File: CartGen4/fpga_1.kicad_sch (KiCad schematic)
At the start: 4 parts, among them U9 LFXP2-8E-5MN132C

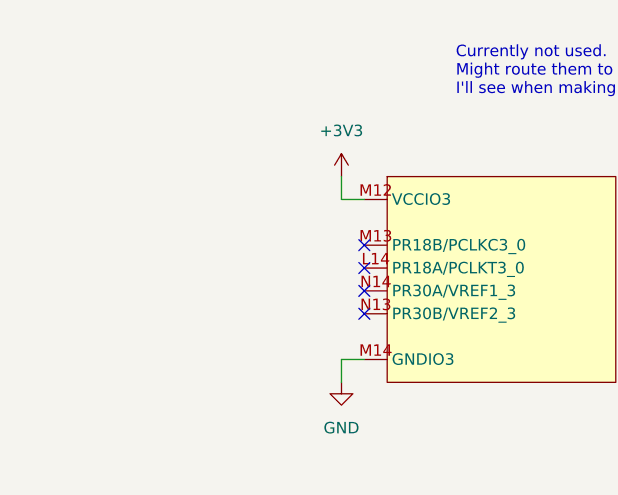
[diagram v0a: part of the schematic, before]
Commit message: Fixed DRC
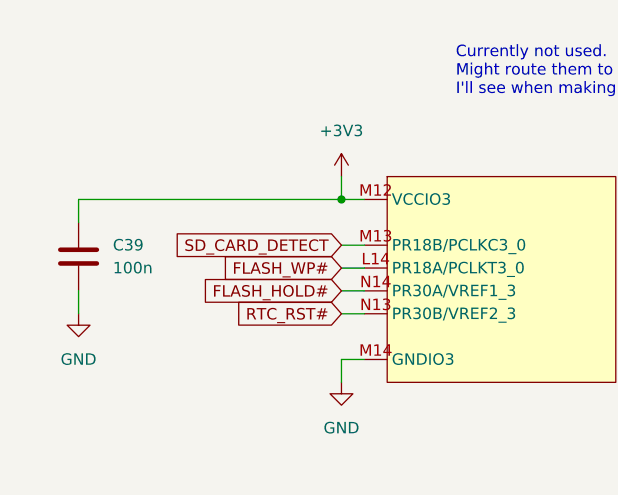
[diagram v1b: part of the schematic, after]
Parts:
- added C39: 100n, symbol Device:C
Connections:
- net +3V3: now also C39.1
- net GND: now also C39.2
- net FLASH_WP#: now reaches U9.L14 (PR18A/PCLKT3_0)
- net SD_CARD_DETECT: now reaches U9.M13 (PR18B/PCLKC3_0)
- net RTC_RST#: now reaches U9.N13 (PR30B/VREF2_3)
- net FLASH_HOLD#: now reaches U9.N14 (PR30A/VREF1_3)
- no-connect marks 8 -> 4
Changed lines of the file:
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@@
   (junction (at 60.96 33.02) (diameter 0) (color 0 0 0 0)
   )
+  (junction (at 50.8 143.51) (diameter 0) (color 0 0 0 0)
+  )
   (junction (at 139.7 48.26) (diameter 0) (color 0 0 0 0)
   )
-  (no_connect (at 53.34 156.21))
   (no_connect (at 119.38 156.21))
   (no_connect (at 119.38 153.67))
   (no_connect (at 119.38 151.13))
   (no_connect (at 119.38 148.59))
-  (no_connect (at 53.34 148.59))
-  (no_connect (at 53.34 151.13))
-  (no_connect (at 53.34 153.67))
   (bus_entry (at 46.99 73.66) (size 2.54 2.54)
     (stroke (width 0) (type default) (color 0 0 0 0))
@@
     (stroke (width 0) (type default) (color 0 0 0 0))
   )
+  (wire (pts (xy 21.59 153.67) (xy 21.59 156.21))
+    (stroke (width 0) (type default) (color 0 0 0 0))
+  )
   (bus (pts (xy 125.73 55.88) (xy 125.73 53.34))
     (stroke (width 0) (type default) (color 0 0 0 0))
@@
     (stroke (width 0) (type default) (color 0 0 0 0))
   )
+  (wire (pts (xy 21.59 143.51) (xy 50.8 143.51))
+    (stroke (width 0) (type default) (color 0 0 0 0))
+  )
   (wire (pts (xy 128.27 81.28) (xy 142.24 81.28))
     (stroke (width 0) (type default) (color 0 0 0 0))
@@
     (stroke (width 0) (type default) (color 0 0 0 0))
   )
+  (wire (pts (xy 50.8 153.67) (xy 53.34 153.67))
+    (stroke (width 0) (type default) (color 0 0 0 0))
+  )
   (wire (pts (xy 128.27 55.88) (xy 142.24 55.88))
     (stroke (width 0) (type default) (color 0 0 0 0))
@@
     (stroke (width 0) (type default) (color 0 0 0 0))
   )
+  (wire (pts (xy 21.59 146.05) (xy 21.59 143.51))
+    (stroke (width 0) (type default) (color 0 0 0 0))
+  )
   (wire (pts (xy 148.59 25.4) (xy 139.7 25.4))
     (stroke (width 0) (type default) (color 0 0 0 0))
@@
     (stroke (width 0) (type default) (color 0 0 0 0))
   )
+  (wire (pts (xy 50.8 151.13) (xy 53.34 151.13))
+    (stroke (width 0) (type default) (color 0 0 0 0))
+  )
   (wire (pts (xy 223.52 69.85) (xy 226.06 69.85))
     (stroke (width 0) (type default) (color 0 0 0 0))
@@
     (stroke (width 0) (type default) (color 0 0 0 0))
   )
+  (wire (pts (xy 50.8 148.59) (xy 53.34 148.59))
+    (stroke (width 0) (type default) (color 0 0 0 0))
+  )
   (bus (pts (xy 125.73 76.2) (xy 125.73 73.66))
     (stroke (width 0) (type default) (color 0 0 0 0))
@@
   )
   (wire (pts (xy 53.34 161.29) (xy 50.8 161.29))
+    (stroke (width 0) (type default) (color 0 0 0 0))
+  )
+  (wire (pts (xy 50.8 156.21) (xy 53.34 156.21))
     (stroke (width 0) (type default) (color 0 0 0 0))
   )
@@
     )
   )
+  (global_label "FLASH_WP#" (shape input) (at 50.8 151.13 180) (fields_autoplaced)
+    (effects (font (size 1.27 1.27)) (justify right))
+    (property "Intersheet References" "${INTERSHEET_REFS}" (id 0) (at 37.6826 151.0506 0)
+      (effects (font (size 1.27 1.27)) (justify right) hide)
+    )
+  )
   (global_label "GB_DATA[0..7]" (shape input) (at 34.29 55.88 180) (fields_autoplaced)
     (effects (font (size 1.27 1.27)) (justify right))
@@
     )
   )
+  (global_label "RTC_RST#" (shape input) (at 50.8 156.21 180) (fields_autoplaced)
+    (effects (font (size 1.27 1.27)) (justify right))
+    (property "Intersheet References" "${INTERSHEET_REFS}" (id 0) (at 39.1945 156.1306 0)
+      (effects (font (size 1.27 1.27)) (justify right) hide)
+    )
+  )
   (global_label "GB_RD#" (shape input) (at 223.52 69.85 180) (fields_autoplaced)
     (effects (font (size 1.27 1.27)) (justify right))
@@
     (effects (font (size 1.27 1.27)) (justify right))
     (property "Intersheet References" "${INTERSHEET_REFS}" (id 0) (at 177.0198 51.9906 0)
+      (effects (font (size 1.27 1.27)) (justify right) hide)
+    )
+  )
+  (global_label "FLASH_HOLD#" (shape input) (at 50.8 153.67 180) (fields_autoplaced)
+    (effects (font (size 1.27 1.27)) (justify right))
+    (property "Intersheet References" "${INTERSHEET_REFS}" (id 0) (at 35.445 153.5906 0)
+      (effects (font (size 1.27 1.27)) (justify right) hide)
+    )
+  )
+  (global_label "SD_CARD_DETECT" (shape input) (at 50.8 148.59 180) (fields_autoplaced)
+    (effects (font (size 1.27 1.27)) (justify right))
+    (property "Intersheet References" "${INTERSHEET_REFS}" (id 0) (at 32.3002 148.6694 0)
       (effects (font (size 1.27 1.27)) (justify right) hide)
     )
@@
     (pin "2")
   )
+  (symbol (lib_id "Device:C") (at 21.59 149.86 0) (unit 1)
+    (in_bom yes) (on_board yes) (fields_autoplaced)
+    (property "Reference" "C39" (id 0) (at 25.4 148.5899 0)
+      (effects (font (size 1.27 1.27)) (justify left))
+    )
+    (property "Value" "100n" (id 1) (at 25.4 151.1299 0)
+      (effects (font (size 1.27 1.27)) (justify left))
+    )
+    (property "Footprint" "" (id 2) (at 22.5552 153.67 0)
+      (effects (font (size 1.27 1.27)) hide)
+    )
+    (property "Datasheet" "~" (id 3) (at 21.59 149.86 0)
+      (effects (font (size 1.27 1.27)) hide)
+    )
+    (pin "1")
+    (pin "2")
+  )
   (symbol (lib_id "power:GND") (at 60.96 86.36 0) (unit 1)
     (in_bom yes) (on_board yes) (fields_autoplaced)
@@
       (effects (font (size 1.27 1.27)) hide)
     )
+    (pin "1")
+  )
+  (symbol (lib_id "power:GND") (at 21.59 156.21 0) (unit 1)
+    (in_bom yes) (on_board yes) (fields_autoplaced)
+    (property "Reference" "#PWR099" (id 0) (at 21.59 162.56 0)
+      (effects (font (size 1.27 1.27)) hide)
+    )
+    (property "Value" "GND" (id 1) (at 21.59 161.29 0))
+    (property "Footprint" "" (id 2) (at 21.59 156.21 0)
+      (effects (font (size 1.27 1.27)) hide)
+    )
+    (property "Datasheet" "" (id 3) (at 21.59 156.21 0)
+      (effects (font (size 1.27 1.27)) hide)
+    )
